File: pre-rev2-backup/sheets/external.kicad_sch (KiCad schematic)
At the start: 39 parts, among them J14 Screw_Terminal_01x02, J5 Screw_Terminal_01x02, Q5 FDS6673BZ_C467780, Q6 FDS6673BZ_C467780, Q7 AO3400A, Q8 AO3400A

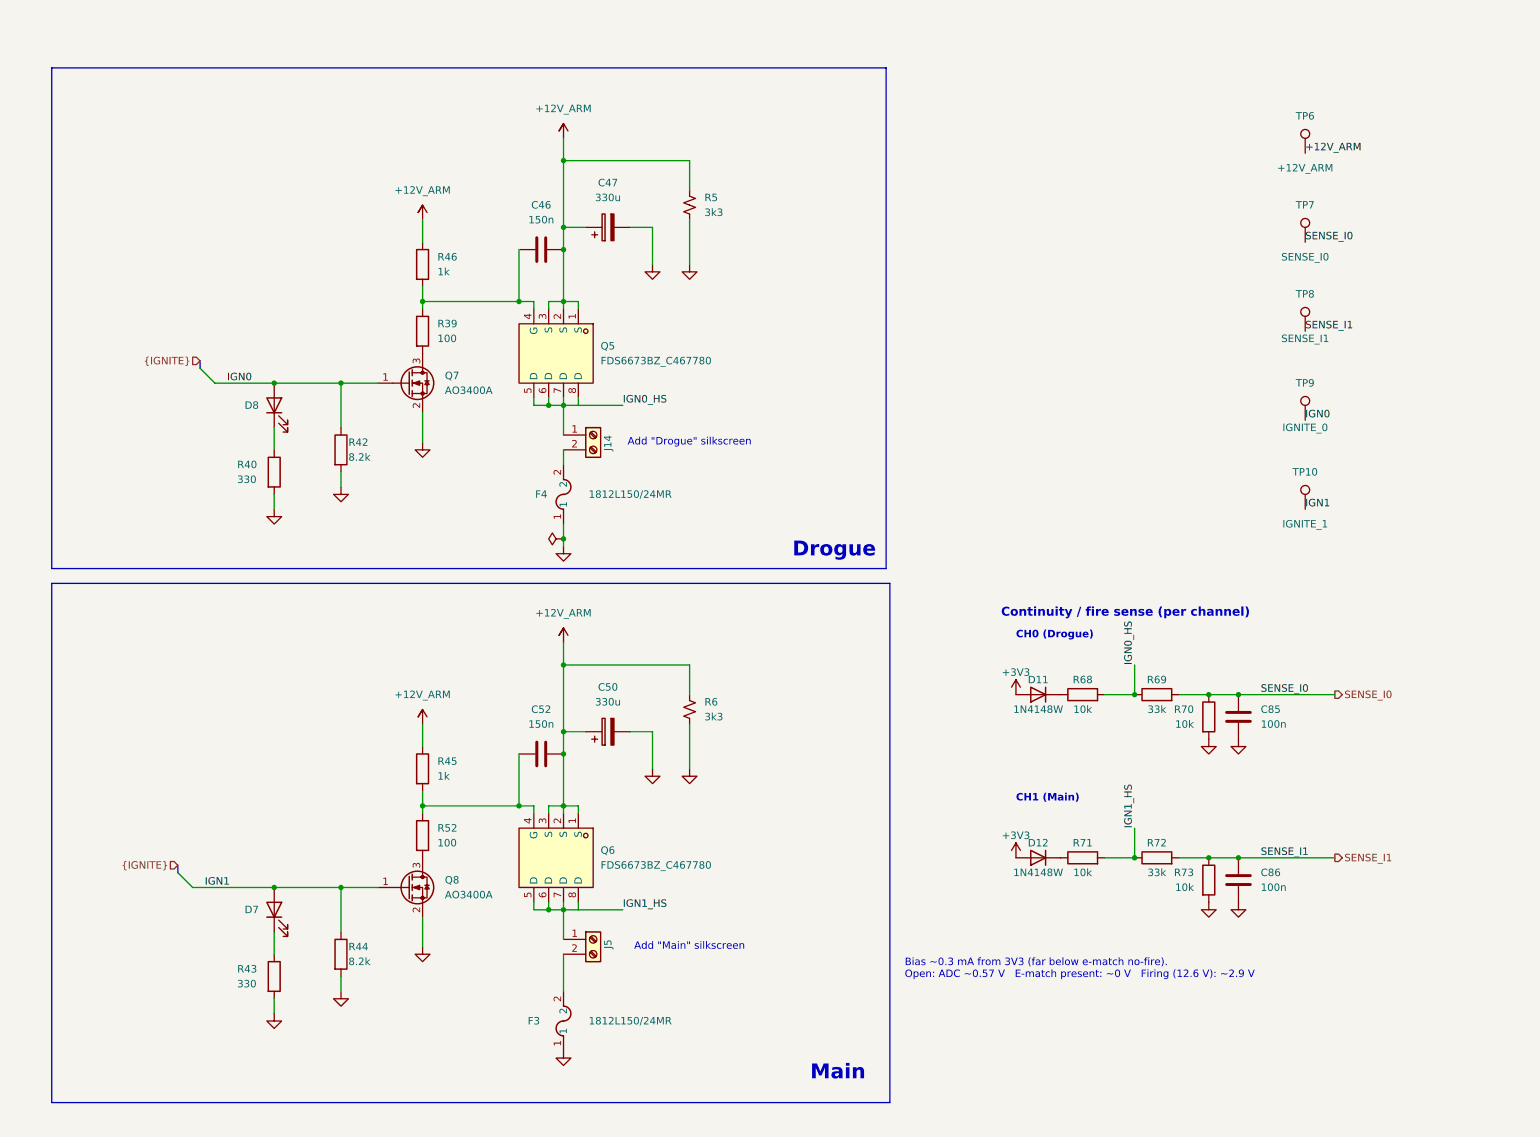
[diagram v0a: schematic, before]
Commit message: Save Aerolotl PCB and schematic progress
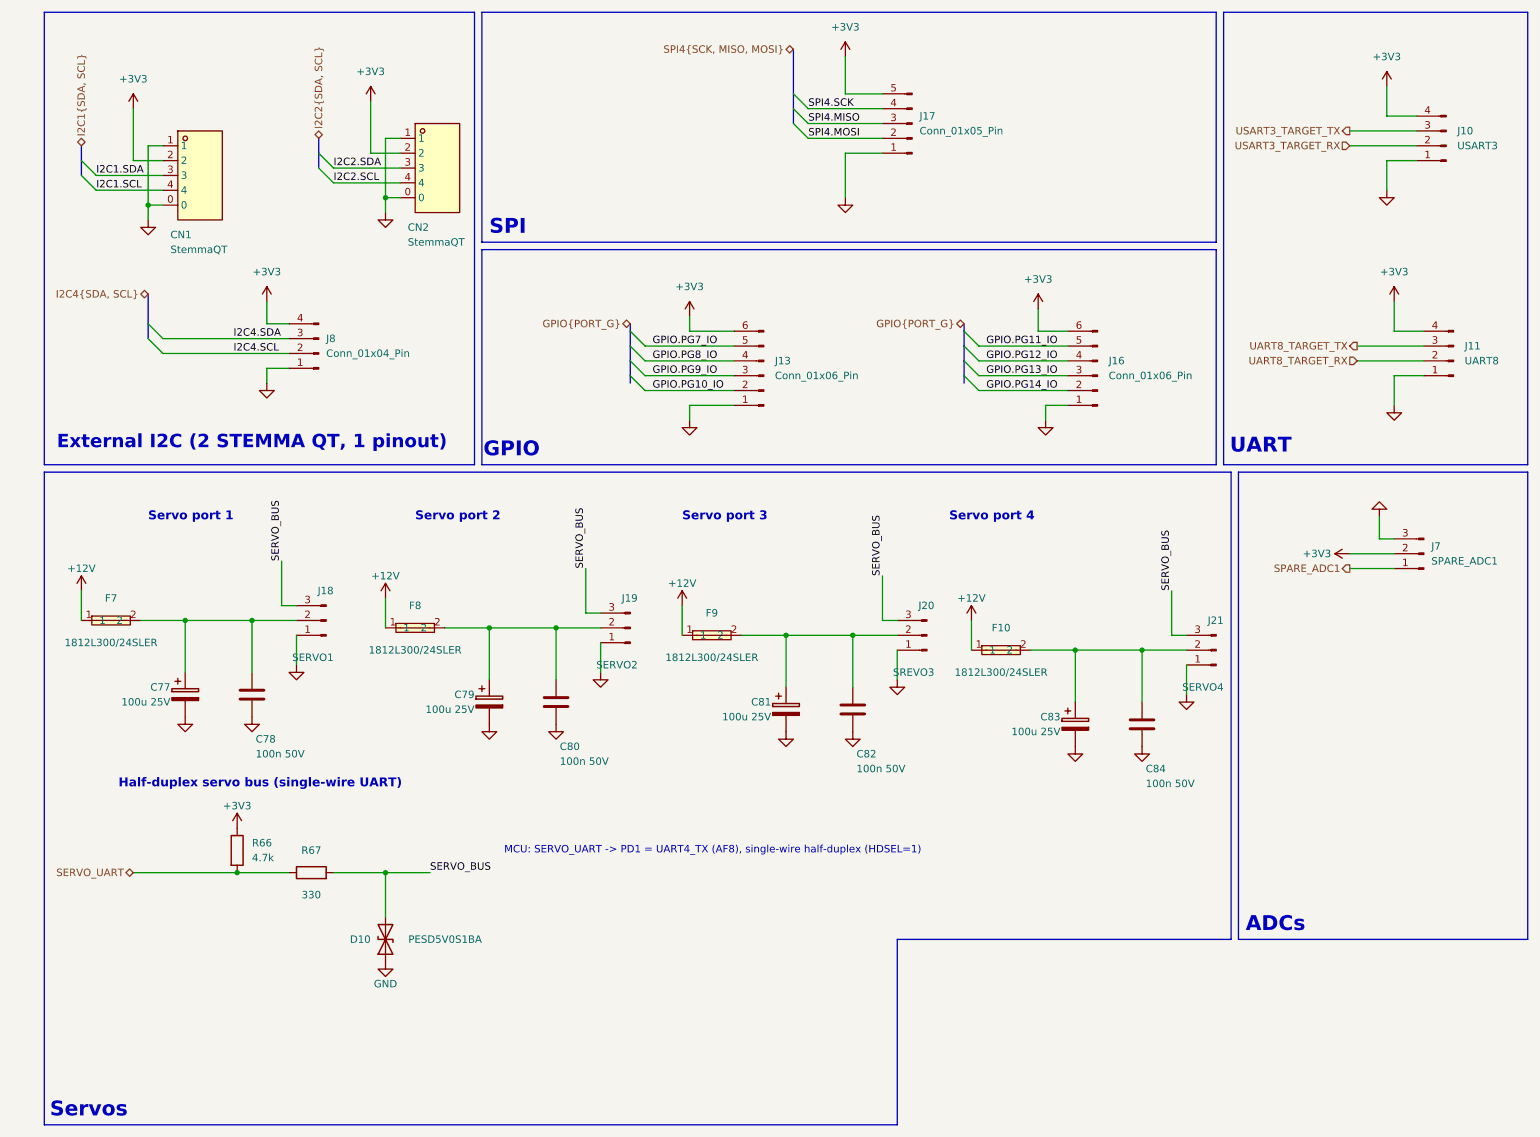
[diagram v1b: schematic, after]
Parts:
- removed C46, C52: 150n, Capacitor_SMD:C_0603_1608Metric, symbol Device:C
- removed C47, C50: 330u, Capacitor_SMD:CP_Elec_8x10, symbol Device:C_Polarized
- removed C85, C86: 100n, Capacitor_SMD:C_0402_1005Metric, symbol Device:C
- removed D11, D12: 1N4148W, Diode_SMD:D_SOD-123, symbol Device:D
- removed D7, D8: LED, LED_SMD:LED_0603_1608Metric, symbol Device:LED
- removed F3, F4: 1812L150/24MR, aerolotl_custom:FUSE_1812L150&slash_24_LTF, symbol aerolotl_custom:1812L150_PTC_Fuse
- removed J14, J5: Screw_Terminal_01x02, TerminalBlock_Phoenix:TerminalBlock_Phoenix_MKDS-1,5-2-5.08_1x02_P5.08mm_Horizontal, symbol Connector:Screw_Terminal_01x02
- removed Q5, Q6: FDS6673BZ_C467780, aerolotl_custom:SOIC-8_L4.9-W3.9-P1.27-LS6.0-BL, symbol aerolotl_custom:FDS6673BZ_C467780
- removed Q7, Q8: AO3400A, Package_TO_SOT_SMD:SOT-23, symbol Transistor_FET:AO3400A
- removed R39, R52: 100, Resistor_SMD:R_0402_1005Metric, symbol Device:R
- removed R40, R43: 330, Resistor_SMD:R_0402_1005Metric, symbol Device:R
- removed R42, R44: 8.2k, Resistor_SMD:R_0402_1005Metric, symbol Device:R
- removed R45, R46: 1k, Resistor_SMD:R_1206_3216Metric, symbol Device:R
- removed R5, R6: 3k3, Resistor_SMD:R_0603_1608Metric, symbol Device:R_Small_US
- removed R68, R70, R71, R73: 10k, Resistor_SMD:R_0402_1005Metric, symbol Device:R
- removed R69, R72: 33k, Resistor_SMD:R_0402_1005Metric, symbol Device:R
- removed TP10: IGNITE_1, TestPoint:TestPoint_Plated_Hole_D2.0mm, symbol Connector:TestPoint
- removed TP6: +12V_ARM, TestPoint:TestPoint_Plated_Hole_D2.0mm, symbol Connector:TestPoint
- removed TP7: SENSE_I0, TestPoint:TestPoint_Plated_Hole_D2.0mm, symbol Connector:TestPoint
- removed TP8: SENSE_I1, TestPoint:TestPoint_Plated_Hole_D2.0mm, symbol Connector:TestPoint
- removed TP9: IGNITE_0, TestPoint:TestPoint_Plated_Hole_D2.0mm, symbol Connector:TestPoint
- added C77, C79, C81, C83: 100u 25V, Capacitor_SMD:CP_Elec_6.3x7.7, symbol Device:C_Polarized
- added C78, C80, C82, C84: 100n 50V, Capacitor_SMD:C_0603_1608Metric, symbol Device:C
- added CN1, CN2: StemmaQT, aerolotl_custom:CONN-SMD_BM04B-SRSS-TB, symbol aerolotl_custom:StemmaQT
- added D10: PESD5V0S1BA, Diode_SMD:D_SOD-323, symbol Device:D_TVS
- added F10, F7, F8, F9: 1812L300/24SLER, Fuse:Fuse_1812_4532Metric, symbol aerolotl_custom:1812L300_24SLER
- added J10: USART3, symbol Connector:Conn_01x04_Pin
- added J11: UART8, symbol Connector:Conn_01x04_Pin
- added J13, J16: Conn_01x06_Pin, symbol Connector:Conn_01x06_Pin
- added J17: Conn_01x05_Pin, symbol Connector:Conn_01x05_Pin
- added J18: SERVO1, Connector_Molex:Molex_SPOX_5267-03A_1x03_P2.50mm_Vertical, symbol Connector:Conn_01x03_Pin
- added J19: SERVO2, Connector_Molex:Molex_SPOX_5267-03A_1x03_P2.50mm_Vertical, symbol Connector:Conn_01x03_Pin
- added J20: SREVO3, Connector_Molex:Molex_SPOX_5267-03A_1x03_P2.50mm_Vertical, symbol Connector:Conn_01x03_Pin
- added J21: SERVO4, Connector_Molex:Molex_SPOX_5267-03A_1x03_P2.50mm_Vertical, symbol Connector:Conn_01x03_Pin
- added J7: SPARE_ADC1, symbol Connector:Conn_01x03_Pin
- added J8: Conn_01x04_Pin, symbol Connector:Conn_01x04_Pin
- added R66: 4.7k, Resistor_SMD:R_0402_1005Metric, symbol Device:R
- added R67: 330, Resistor_SMD:R_0402_1005Metric, symbol Device:R
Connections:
- net +3V3: now also CN1.2, CN2.2, J10.4 (Pin_4), J11.4 (Pin_4), J13.6 (Pin_6), J16.6 (Pin_6), J17.5 (Pin_5), J7.2 (Pin_2), J8.4 (Pin_4), R66.1
- net GND: now also C77.2, C78.2, C79.2, C80.2, C81.2, C82.2, C83.2, C84.2, CN1.0, CN1.1, CN2.0, CN2.1, D10.1 (A1), J10.1 (Pin_1), J11.1 (Pin_1), J13.1 (Pin_1), J16.1 (Pin_1), J17.1 (Pin_1), J18.1 (Pin_1), J19.1 (Pin_1), J20.1 (Pin_1), J21.1 (Pin_1), J7.3 (Pin_3), J8.1 (Pin_1)
- new net: C81.1, C82.1, F9.2, J20.2 (Pin_2)
- new net: C79.1, C80.1, F8.2, J19.2 (Pin_2)
- new net: C77.1, C78.1, F7.2, J18.2 (Pin_2)
- new net: C83.1, C84.1, F10.2, J21.2 (Pin_2)
- new net +12V: F10.1, F7.1, F8.1, F9.1
- new net GPIO.PG10_IO: J13.2 (Pin_2)
- new net GPIO.PG11_IO: J16.5 (Pin_5)
- new net GPIO.PG12_IO: J16.4 (Pin_4)
- new net GPIO.PG13_IO: J16.3 (Pin_3)
- new net GPIO.PG14_IO: J16.2 (Pin_2)
- new net GPIO.PG7_IO: J13.5 (Pin_5)
- new net GPIO.PG8_IO: J13.4 (Pin_4)
- new net GPIO.PG9_IO: J13.3 (Pin_3)
- new net I2C1.SCL: CN1.4
- new net I2C1.SDA: CN1.3
- new net I2C2.SCL: CN2.4
- new net I2C2.SDA: CN2.3
- new net I2C4.SCL: J8.2 (Pin_2)
- new net I2C4.SDA: J8.3 (Pin_3)
- new net SERVO_BUS: D10.2 (A2), J18.3 (Pin_3), J19.3 (Pin_3), J20.3 (Pin_3), J21.3 (Pin_3), R67.2
- new net SERVO_UART: R66.2, R67.1
- new net SPARE_ADC1: J7.1 (Pin_1)
- new net SPI4.MISO: J17.3 (Pin_3)
- new net SPI4.MOSI: J17.2 (Pin_2)
- new net SPI4.SCK: J17.4 (Pin_4)
- new net UART8_TARGET_RX: J11.2 (Pin_2)
- new net UART8_TARGET_TX: J11.3 (Pin_3)
- new net USART3_TARGET_RX: J10.2 (Pin_2)
- new net USART3_TARGET_TX: J10.3 (Pin_3)
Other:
- note added: "ADCs"
- note added: "External I2C (2 STEMMA QT, 1 pinout)"
- note added: "GPIO"
- note added: "Half-duplex servo bus (single-wire UART)"
- note added: "MCU: SERVO_UART -> PD1 = UART4_TX (AF8), single-wire half-duplex (HDSEL=1)"
- note added: "SPI"
- note added: "Servo port 1"
- note added: "Servo port 2"
- note added: "Servo port 3"
- note added: "Servo port 4"
- note added: "Servos"
- note added: "UART"
- note removed: "Add "Drogue" silkscreen"
- note removed: "Add "Main" silkscreen"
- note removed: "Bias ~0.3 mA from 3V3 (far below e-match no-fire). Open: ADC ~0.57 V E-match present: ~0 V Firing (12.6 V): ~2.9 V"
- note removed: "CH0 (Drogue)"
- note removed: "CH1 (Main)"
- note removed: "Continuity / fire sense (per channel)"
- note removed: "Drogue"
- note removed: "Main"
